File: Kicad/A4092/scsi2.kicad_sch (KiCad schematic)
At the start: 33 parts, among them U9 LSI53C770 SCSI Host Controller

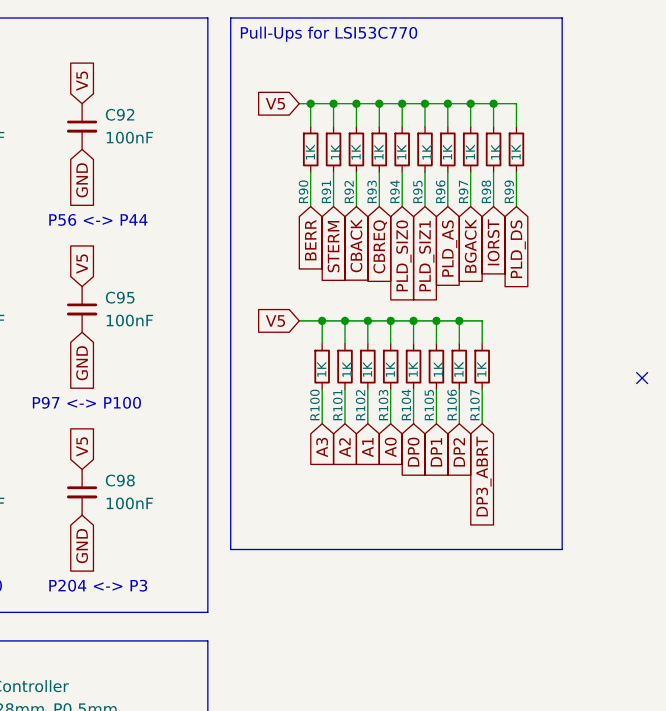
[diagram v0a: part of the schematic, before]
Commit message: Clean up pull-up resistors
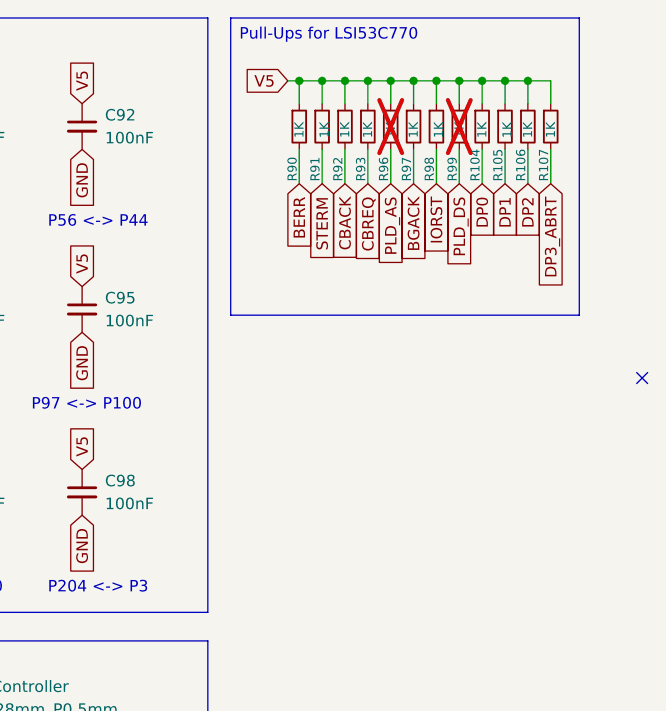
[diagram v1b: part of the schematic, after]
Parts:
- removed R100, R101, R102, R103, R94, R95: 1K, Resistor_SMD:R_0603_1608Metric_Pad0.98x0.95mm_HandSolder, symbol Device:R_Small
- R96, R99: now not fitted
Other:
- title: A4092 -> Cheetah UW
- moved on the sheet: R104, R105, R106, R107, R90, R91, R92, R93, R97, R98
